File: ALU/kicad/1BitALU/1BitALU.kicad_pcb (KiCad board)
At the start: 2 copper layers, 158.8 x 158.8 mm, 55 parts, among them P1 CONN_6, P2 CONN_2, P3 Power, U1 xor3a, U10 and3a, U11 or2a, U12 and3b, U13 inv3b, U14 and3c, U15 or3a, U16 xor1b, U17 xor1a, U18 xor2b, U19 and4a, U2 and2a, U20 xor2a, U21 and4b, U22 and4c, U23 or3b, U24 and5a, U25 and5b, U26 inv5c, U27 and5c, U28 or3c, U29 and6a, U3 xor3b, U30 inv6b, U31 and6b, U32 inv6c, U33 and6c, U34 or3d, U4 and2b, U5 or1b, U6 and1a, U7 and1b, U8 or1a, U9 or2b

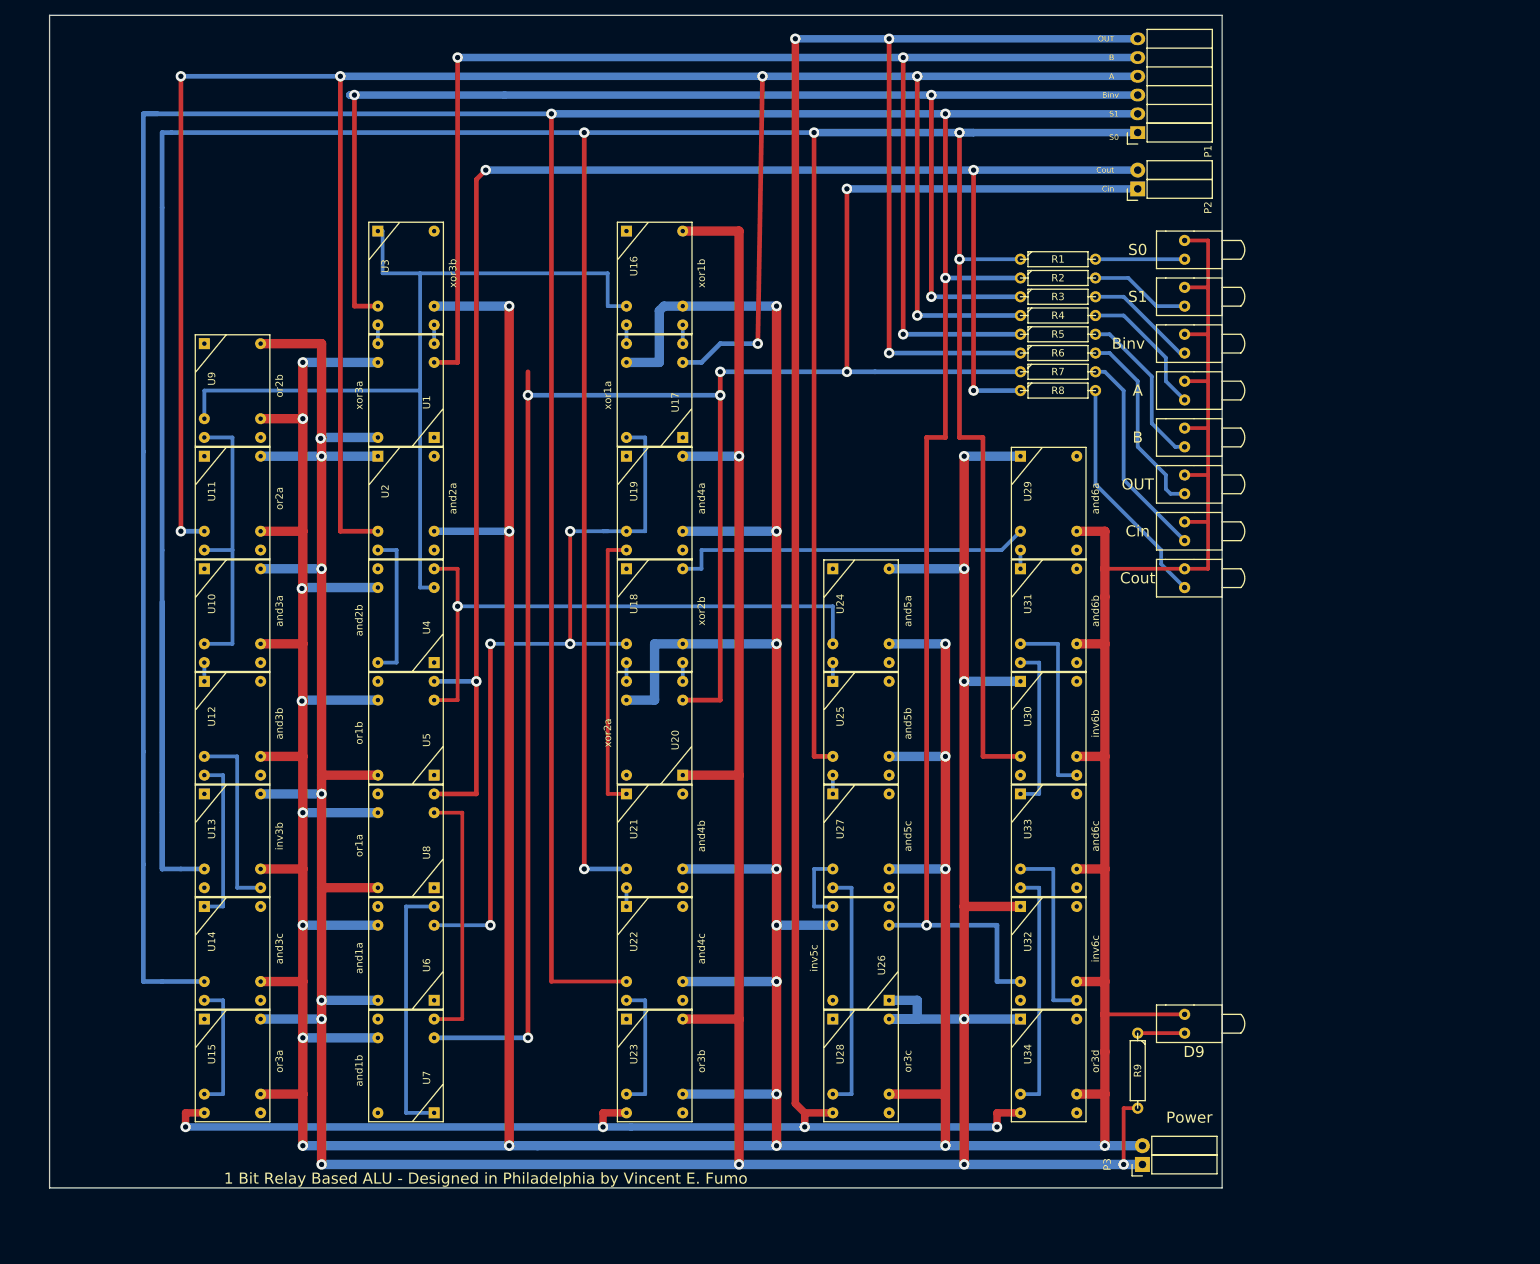
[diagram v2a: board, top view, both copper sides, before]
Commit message: interim version
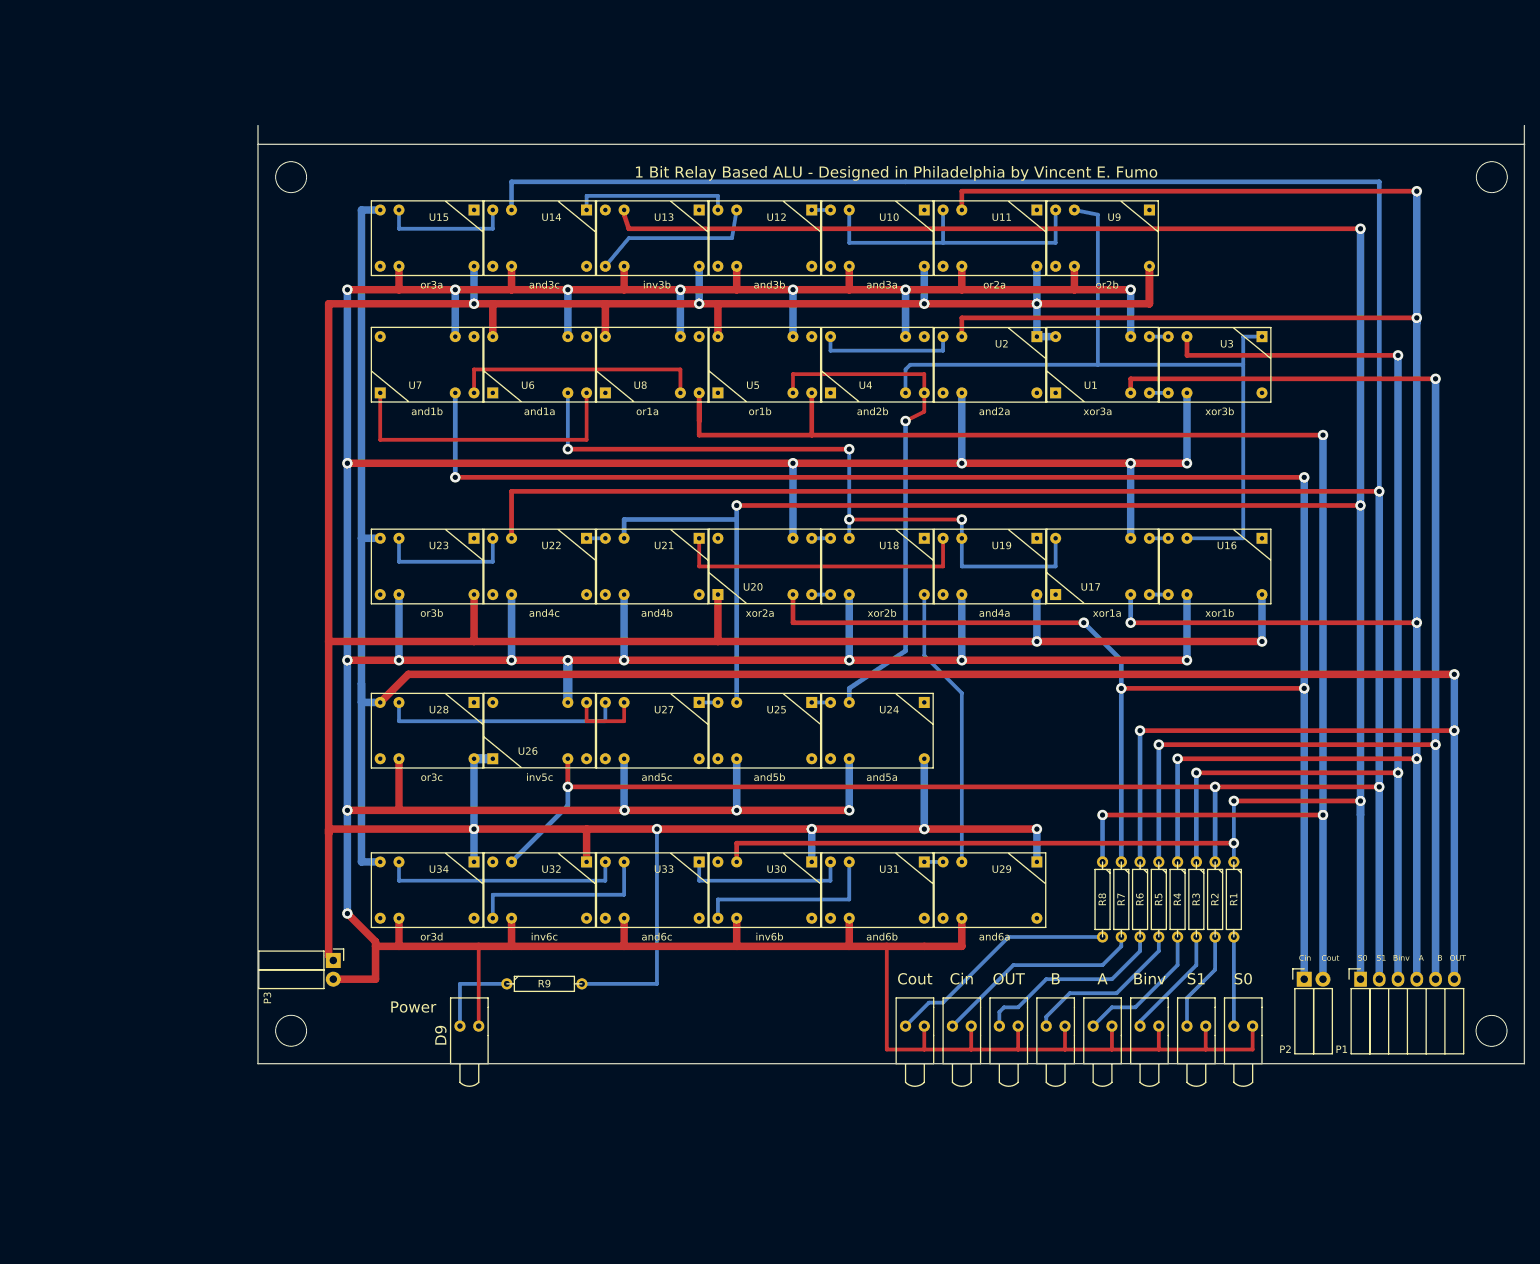
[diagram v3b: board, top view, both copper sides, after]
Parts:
- moved U9 120.8 mm to (166.7, 47.9), turned to 180 degrees
- moved P1 118.5 mm to (195.3, 144.5), turned to 0 degrees
- moved U3 114.2 mm to (181.9, 65.1), turned to 180 degrees
- moved P3 113.0 mm to (56.2, 141.9), turned to 270 degrees
- moved D1 109.5 mm to (183.2, 150.8), turned to 270 degrees
- moved P2 109.3 mm to (187.6, 144.5), turned to 0 degrees
- moved U11 108.2 mm to (151.4, 47.9), turned to 180 degrees
- moved U15 105.9 mm to (75.2, 47.9), turned to 180 degrees
- moved U7 105.1 mm to (62.5, 57.5), turned to 0 degrees
- moved D2 102.7 mm to (176.8, 150.8), turned to 270 degrees
- moved U10 98.7 mm to (136.2, 47.9), turned to 180 degrees
- moved U14 97.3 mm to (90.5, 47.9), turned to 180 degrees
- moved D3 96.2 mm to (170.5, 150.8), turned to 270 degrees
- moved U12 93.4 mm to (121.0, 47.9), turned to 180 degrees
- moved D9 93.1 mm to (78.4, 150.8), turned to 270 degrees
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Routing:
- net S0 Bus: track 605.2 -> 429.4 mm, vias 5 -> 6
- net GND: track 1060.7 -> 890.6 mm, vias 24 -> 25
- net +5V: track 625.2 -> 570.5 mm, vias 15 -> 11
- net S1 Bus: track 537.8 -> 494.0 mm
- net OUT: track 382.8 -> 349.6 mm, vias 7 -> 3
- net A: track 354.8 -> 324.5 mm, vias 7 -> 6
- net Binv: track 178.4 -> 154.9 mm
- net Cin: track 283.2 -> 296.7 mm, vias 6 -> 5
- net Cout: track 220.9 -> 208.3 mm, vias 4 -> 3
- net B: track 189.9 -> 177.8 mm
- net B Actual: track 121.3 -> 110.2 mm
- net ADD Out: track 49.3 -> 38.3 mm
- net AND Out: track 80.0 -> 70.4 mm
- net XOR Out: track 105.4 -> 95.9 mm
- net Net-(D9-Pad1): track 6.35 -> 12.1 mm
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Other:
- board size 158.8 x 158.8 mm -> 171.5 x 127 mm
- net class Power: clearance 0.635 -> 0.508; trace_width 1.27 -> 1.016
